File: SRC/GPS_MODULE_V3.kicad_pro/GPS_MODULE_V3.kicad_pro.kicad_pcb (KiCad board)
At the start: 4 copper layers, 53.7 x 41 mm, 143 parts, among them J1 Input, J2 Conn_02x02_Odd_Even, J3 nano_sim, J5 Conn_02x03_Odd_Even, Q1 SSM3J328R-HXY, Q2 BSN20, Q3 BSN20, Q5 2N7002, Q6 2N7002, Q7 2N7002, Q8 2N7002, Q9 2N7002, U1 SY8089AAAC, U2 STM32F103C8Tx, U3 SIM7000E, U4 MAX485E, U7 ATA6561-GAQW-N, U8 W25Q32JVSS, Y1 8MHz, Y2 32.678KHz

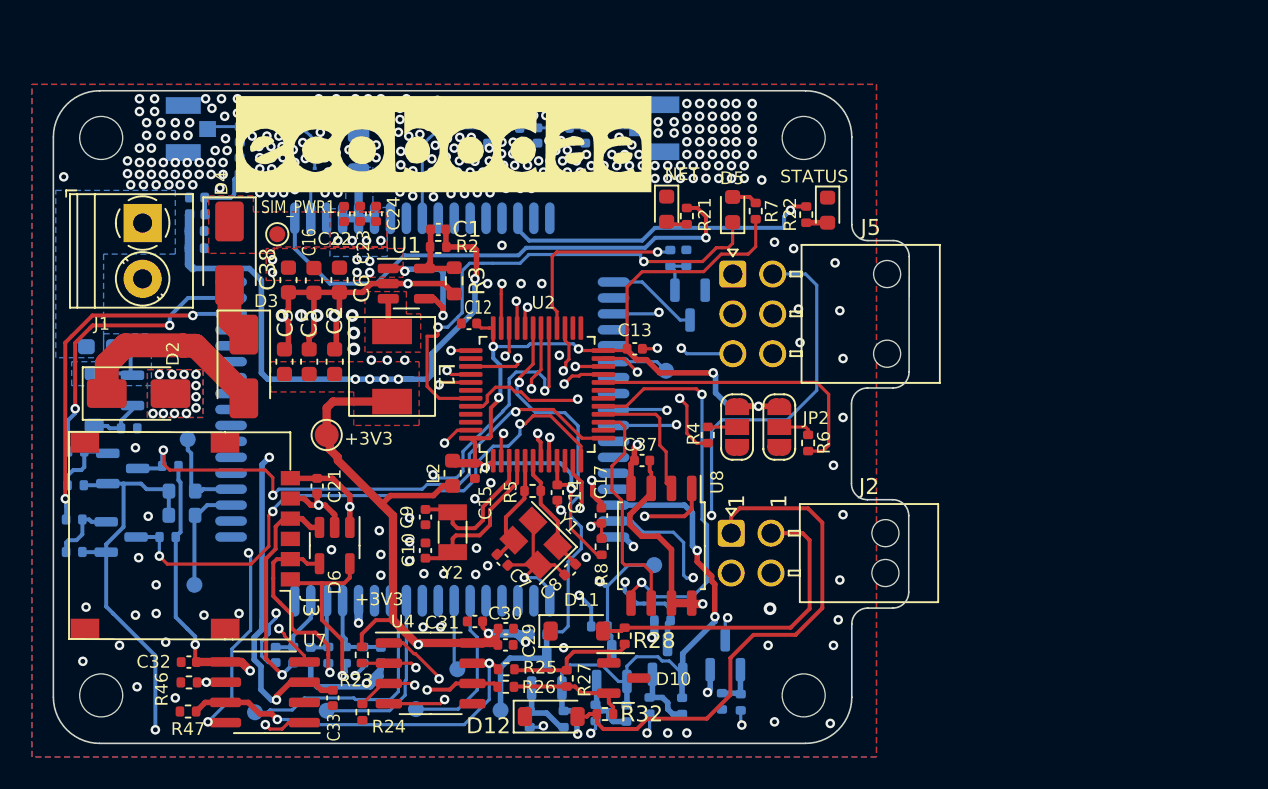
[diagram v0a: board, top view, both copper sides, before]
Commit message: updates on BOM, CPL and gerbers
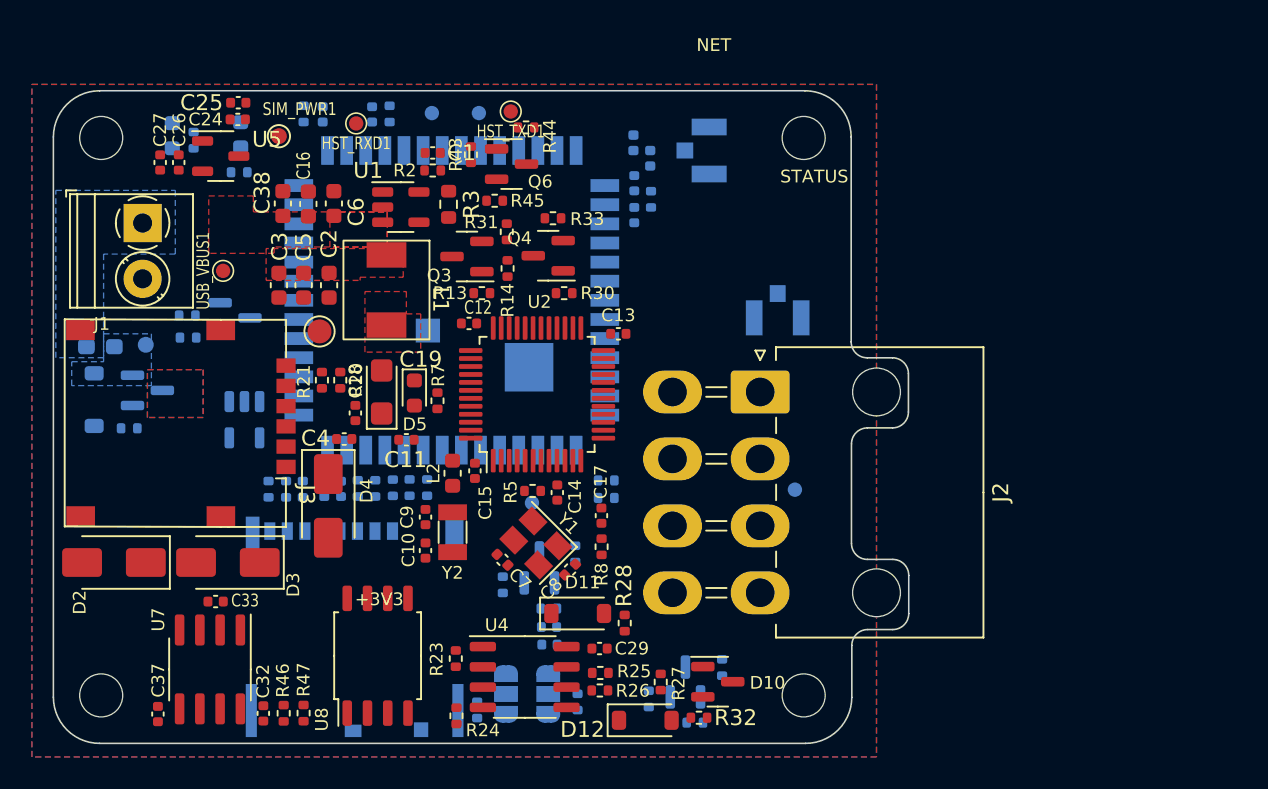
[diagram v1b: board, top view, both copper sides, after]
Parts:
- removed BOOT_CFG1: BOOT_CFG, TestPoint:TestPoint_Pad_D1.0mm
- removed C35: 10n, Capacitor_SMD:C_0402_1005Metric
- removed C36: 1n, Capacitor_SMD:C_0402_1005Metric
- removed FL1: B39162B8813P810, Filter:Filter_1109-5_1.1x0.9mm
- removed the G*** at (247.8, 69.3)
- removed J5: Conn_02x03_Odd_Even, Connector_Molex:Molex_Nano-Fit_105314-xx06_2x03_P2.50mm_Horizontal
- removed L4: 27nH, Inductor_SMD:L_0402_1005Metric
- removed L5: 100mHz 150/200R, Inductor_SMD:L_0402_1005Metric
- removed MDM_LOG_TX1: MDM_LOG_TX, TestPoint:TestPoint_Pad_D1.0mm
- removed Q8, Q9: 2N7002, Package_TO_SOT_SMD:SOT-23
- removed SIM_RX1: Sim_RX, TestPoint:TestPoint_Pad_D1.0mm
- removed SIM_TX1: Sim_TX, TestPoint:TestPoint_Pad_D1.0mm
- added C11: 10u, Capacitor_SMD:C_0402_1005Metric, F.Cu at (245.5, 87.9)
- added C4: 1u, Capacitor_SMD:C_0402_1005Metric, F.Cu at (241.6, 87.8)
- added G***: LOGO, MACHADA_footprints:ECOBODDA_SMALL, B.Cu at (230.8, 97.7)
- added HST_RXD1: HST_RXD, brilliant-kicad-library:TestPoint_Pad_D0.9mm, F.Cu at (242.3, 68.0)
- added HST_TXD1: HST_TXD, brilliant-kicad-library:TestPoint_Pad_D0.9mm, F.Cu at (252.1, 67.3)
- added J4: Micro_SD_Card, MACHADA_footprints:MOLEX_503398-1892, B.Cu at (242.2, 99.2)
- added Q4: 2N7002, Package_TO_SOT_SMD:SOT-23, F.Cu at (254.4, 76.3)
- added R36: 1K, Resistor_SMD:R_0402_1005Metric, B.Cu at (260.7, 104.2)
- added R48: 10K, Resistor_SMD:R_0402_1005Metric, B.Cu at (254.4, 98.5)
- added R49: 10K, Resistor_SMD:R_0402_1005Metric, B.Cu at (256.1, 95.1)
- added R50: 1K, Resistor_SMD:R_0402_1005Metric, B.Cu at (251.6, 97.0)
- added U5: XC6206PxxxMR, Package_TO_SOT_SMD:SOT-23-3, F.Cu at (233.8, 70.1)
- C18: value 22p -> 10u; moved to F.Cu
- C19: value 22p -> 100u; footprint Capacitor_SMD:C_0402_1005Metric -> Capacitor_Tantalum_SMD:CP_EIA-3216-18_Kemet-A; moved to F.Cu
- C20: value 22p -> 1u
- C21: value 100n -> 22p; moved to B.Cu
- C22: value 1u -> 22p; moved to B.Cu
- C23: value 10u -> 22p; moved to B.Cu
- C24: value 10u -> 0.1u
- C25: value 100u -> 1u; footprint Capacitor_Tantalum_SMD:CP_EIA-3216-18_Kemet-A -> Capacitor_SMD:C_0402_1005Metric; moved to F.Cu
- C26: value 0.3p -> 0.1u; moved to F.Cu
- C27: value ~ -> 1u; moved to F.Cu
- C28: value ~ -> 0.1u
- C30, C31, JP1, JP2, R22, R4, R6: moved to B.Cu
- D+1, D-1, SIM_I2C_SCL1, SIM_I2C_SDA1: footprint TestPoint:TestPoint_Pad_D1.0mm -> brilliant-kicad-library:TestPoint_Pad_D0.9mm
- D6: value SP0504BAHT -> LXES15AAA1-153; footprint Package_TO_SOT_SMD:SOT-23-5 -> Diode_SMD:D_0402_1005Metric; moved to B.Cu
- D7: value ORANGE -> SP0504BAHT; footprint LED_SMD:LED_0603_1608Metric -> Package_TO_SOT_SMD:SOT-23-5; moved to B.Cu
- D8: value BLUE -> ORANGE; moved to B.Cu
- D9: value LXES15AAA1-153 -> BLUE; footprint Diode_SMD:D_0402_1005Metric -> LED_SMD:LED_0603_1608Metric
- J2: value Conn_02x02_Odd_Even -> Conn_02x04_Odd_Even; footprint Connector_Molex:Molex_Nano-Fit_105314-xx04_2x02_P2.50mm_Horizontal -> Connector_Molex:Molex_Mini-Fit_Jr_5569-08A2_2x04_P4.20mm_Horizontal
- L3: value 1uH -> 82nH
- Q3, Q6, R43, R44: moved to F.Cu
- R10: value 1k -> 10K
- R12: value 10K -> 1k
- R13: value 22R -> 1k; moved to F.Cu
- R14: value 22R -> 10K; moved to F.Cu
- R15: value 22R -> 2.2K
- R16: value 10K -> 2.2K
- R17, R18: value 2.2K -> 22R; footprint Resistor_SMD:R_0603_1608Metric -> Resistor_SMD:R_0402_1005Metric
- R19: value 0R -> 22R
- R20: value 10R -> 200K; moved to F.Cu
- R21: value 390R -> 100K
- R29: value 1K -> 390R
- R30, R31: value 1K -> 10K; moved to F.Cu
- R33, R45: value 10K -> 1K; moved to F.Cu
- R37, R38, R39, R42: value 10K -> 10k
- R40, R41: value 1K -> 10k
- U3: value SIM7000E -> A9G_MODULE; footprint Lib:SIMCON_SIM7000E -> MACHADA_footprints:A9G_MODULE
- USB_VBUS1: footprint TestPoint:TestPoint_Pad_D1.0mm -> brilliant-kicad-library:TestPoint_Pad_D0.9mm; moved to F.Cu
- moved R10 42.4 mm to (231.8, 80.1), turned to 0 degrees
- moved D8 41.4 mm to (230.8, 68.8)
- moved R29 40.6 mm to (235.0, 71.1), turned to 180 degrees
- moved D-1 40.1 mm to (250.1, 67.4), turned to 90 degrees
- moved AE2 39.1 mm to (268.8, 80.2), turned to 0 degrees
- moved R22 38.7 mm to (232.2, 69.1)
- moved SIM_I2C_SDA1 38.2 mm to (269.9, 91.0)
- moved D+1 38.1 mm to (247.1, 67.4), turned to 90 degrees
- moved C20 35.6 mm to (259.8, 73.8)
- moved R17 34.7 mm to (260.9, 72.8), turned to -90 degrees
- moved C37 34.3 mm to (229.9, 105.1), turned to -90 degrees
- moved R44 34.2 mm to (253.0, 68.3), turned to 0 degrees
- moved Q6 32.6 mm to (252.1, 70.6), turned to 0 degrees
- moved R43 32.3 mm to (249.6, 70.0), turned to -90 degrees
- moved R33 31.4 mm to (254.7, 74.0), turned to 0 degrees
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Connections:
- C18 pad 1: /SIM7000E_GPRS_SIM MODULE/Sim_DIO -> 4.2V_SIMPWR
- C19 pad 1: /SIM7000E_GPRS_SIM MODULE/Sim_CLK -> 4.2V_SIMPWR
- C20 pad 1: /SIM7000E_GPRS_SIM MODULE/Sim_RST -> /A9G_GSM_GPRS_MODULE/VIO
- C21 pad 1: /SIM7000E_GPRS_SIM MODULE/V_Sim -> /A9G_GSM_GPRS_MODULE/Sim_DIO
- C22 pad 1: 4.2V_SIMPWR -> /A9G_GSM_GPRS_MODULE/Sim_CLK
- C23 pad 1: 4.2V_SIMPWR -> /A9G_GSM_GPRS_MODULE/Sim_RST
- C26 pad 1: GND -> 2V8
- C26 pad 2: /SIM7000E_GPRS_SIM MODULE/RF_ANT -> GND
- C27 pad 1: GND -> 2V8
- C27 pad 2: Net-(C27-Pad2) -> GND
- C28 pad 1: GND -> /A9G_GSM_GPRS_MODULE/TF_CARD_CONN/2V8
- C28 pad 2: Net-(AE1-A) -> GND
- C34 pad 1: +3V3 -> /A9G_GSM_GPRS_MODULE/TF_CARD_CONN/2V8
- D+1 pad 1: Net-(U3-USB_DP) -> Net-(U3-USB_P)
- D-1 pad 1: Net-(U3-USB_DM) -> Net-(U3-USB_N)
- D6 pad 1: /SIM7000E_GPRS_SIM MODULE/V_Sim -> GND
- D6 pad 2: GND -> Net-(AE1-A)
- D7 pad 1: GND -> /A9G_GSM_GPRS_MODULE/V_Sim
- D7 pad 2: Net-(D7-A) -> GND
- D9 pad 2: Net-(AE1-A) -> Net-(D9-A)
- J2 pad 1: /RS485_MAX485/A -> GND
- J2 pad 3: /RS485_MAX485/B -> /RS485_MAX485/A
- J2 pad 4: GND -> /STM32F103C8T6_MCU/SW0
- J3 pad C1: /SIM7000E_GPRS_SIM MODULE/V_Sim -> /A9G_GSM_GPRS_MODULE/V_Sim
- L3 pad 1: /SIM7000E_GPRS_SIM MODULE/RF_ANT -> GND
- L3 pad 2: Net-(C27-Pad2) -> Net-(AE1-A)
- Q5 pad 1: /SIM7000E_GPRS_SIM MODULE/VDD_EXT -> 2V8
- Q5 pad 3: /STM32F103C8T6_MCU/TX1 -> /STM32F103C8T6_MCU/RX2
- Q6 pad 1: /SIM7000E_GPRS_SIM MODULE/VDD_EXT -> 2V8
- Q6 pad 3: /SIM7000E_GPRS_SIM MODULE/SIM_DTR -> /STM32F103C8T6_MCU/TX2
- Q7 pad 1: /SIM7000E_GPRS_SIM MODULE/VDD_EXT -> 2V8
- Q7 pad 3: /STM32F103C8T6_MCU/RX1 -> /STM32F103C8T6_MCU/TX1
- R10 pad 1: /SIM7000E_GPRS_SIM MODULE/Sim_Reset -> GND
- R10 pad 2: Net-(Q3-G) -> Net-(Q2-G)
- R11 pad 1: GND -> Net-(Q3-D)
- R11 pad 2: Net-(Q2-G) -> /A9G_GSM_GPRS_MODULE/VIO
- R12 pad 1: GND -> /A9G_GSM_GPRS_MODULE/IO29
- R12 pad 2: Net-(Q3-G) -> Net-(Q3-D)
- R13 pad 1: /SIM7000E_GPRS_SIM MODULE/Sim_RST -> /A9G_GSM_GPRS_MODULE/PWRKEY
- R13 pad 2: Net-(J3-RST) -> Net-(Q3-G)
- R14 pad 1: /SIM7000E_GPRS_SIM MODULE/Sim_CLK -> GND
- R14 pad 2: Net-(J3-CLK) -> Net-(Q3-G)
- R15 pad 1: /SIM7000E_GPRS_SIM MODULE/Sim_DIO -> Net-(U3-I2C2_SCL/IO19)
- R15 pad 2: Net-(J3-I/O) -> /A9G_GSM_GPRS_MODULE/VIO
- R16 pad 1: /SIM7000E_GPRS_SIM MODULE/Sim_DIO -> Net-(U3-I2C2_SDA/IO20)
- R16 pad 2: /SIM7000E_GPRS_SIM MODULE/V_Sim -> /A9G_GSM_GPRS_MODULE/VIO
- R17 pad 1: Net-(U3-I2C_SCL) -> /A9G_GSM_GPRS_MODULE/Sim_RST
- R17 pad 2: /SIM7000E_GPRS_SIM MODULE/VDD_EXT -> Net-(J3-RST)
- R18 pad 1: Net-(U3-I2C_SDA) -> /A9G_GSM_GPRS_MODULE/Sim_CLK
- R18 pad 2: /SIM7000E_GPRS_SIM MODULE/VDD_EXT -> Net-(J3-CLK)
- R19 pad 1: Net-(C27-Pad2) -> /A9G_GSM_GPRS_MODULE/Sim_DIO
- R19 pad 2: Net-(AE1-A) -> Net-(J3-I/O)
- R20 pad 1: Net-(L4-Pad1) -> Net-(U3-ADC0)
- R20 pad 2: /SIM7000E_GPRS_SIM MODULE/gps_VDD -> 4.2V_SIMPWR
- R21 pad 1: /SIM7000E_GPRS_SIM MODULE/NETLIGHT -> GND
- R21 pad 2: Net-(D7-A) -> Net-(U3-ADC0)
- R22 pad 1: /SIM7000E_GPRS_SIM MODULE/STATUS -> /A9G_GSM_GPRS_MODULE/GPRS_NET-STATUS
- R29 pad 1: /SIM7000E_GPRS_SIM MODULE/MOSFET_LOGIC_LEVEL_TRANSLATOR/LOW_SIDE_SIM_RXD_LOGIC -> /A9G_GSM_GPRS_MODULE/GPS POSITION
- R29 pad 2: Net-(Q5-S) -> Net-(D9-A)
- R30 pad 1: /SIM7000E_GPRS_SIM MODULE/MOSFET_LOGIC_LEVEL_TRANSLATOR/LOW_SIDE_SIM_DTR_LOGIC -> 2V8
- R30 pad 2: Net-(Q6-S) -> Net-(Q4-S)
- R31 pad 1: /SIM7000E_GPRS_SIM MODULE/MOSFET_LOGIC_LEVEL_TRANSLATOR/LOW_SIDE_SIM_TXD_LOGIC -> +3V3
- R31 pad 2: Net-(Q7-S) -> /STM32F103C8T6_MCU/RX1
- R33 pad 1: /SIM7000E_GPRS_SIM MODULE/VDD_EXT -> /A9G_GSM_GPRS_MODULE/MOSFET_LOGIC_LEVEL_TRANSLATOR9/LOW_SIDE_LOGIC_SIGNAL
- R33 pad 2: Net-(Q5-S) -> Net-(Q4-S)
- R34 pad 1: /SIM7000E_GPRS_SIM MODULE/VDD_EXT -> 2V8
- R34 pad 2: Net-(Q6-S) -> Net-(Q5-S)
- R35 pad 1: /SIM7000E_GPRS_SIM MODULE/VDD_EXT -> +3V3
- R35 pad 2: Net-(Q7-S) -> /STM32F103C8T6_MCU/RX2
- R37 pad 1: +3V3 -> /A9G_GSM_GPRS_MODULE/TF_CARD_CONN/2V8
- R37 pad 2: /STM32F103C8T6_MCU/TX1 -> /A9G_GSM_GPRS_MODULE/TF_CARD_CONN/SD_D2
- R38 pad 1: +3V3 -> /A9G_GSM_GPRS_MODULE/TF_CARD_CONN/2V8
- R38 pad 2: /SIM7000E_GPRS_SIM MODULE/SIM_DTR -> /A9G_GSM_GPRS_MODULE/TF_CARD_CONN/SD_D3
- R39 pad 1: +3V3 -> /A9G_GSM_GPRS_MODULE/TF_CARD_CONN/2V8
- R39 pad 2: /STM32F103C8T6_MCU/RX1 -> /A9G_GSM_GPRS_MODULE/TF_CARD_CONN/SD_CMD
- R40 pad 1: /SIM7000E_GPRS_SIM MODULE/GPS_RXD_ -> /A9G_GSM_GPRS_MODULE/TF_CARD_CONN/2V8
- R40 pad 2: Net-(Q8-S) -> /A9G_GSM_GPRS_MODULE/TF_CARD_CONN/SD_D0
- R41 pad 1: /SIM7000E_GPRS_SIM MODULE/GPS_TXD_ -> /A9G_GSM_GPRS_MODULE/TF_CARD_CONN/2V8
- R41 pad 2: Net-(Q9-S) -> /A9G_GSM_GPRS_MODULE/TF_CARD_CONN/SD_D1
- R42 pad 1: /SIM7000E_GPRS_SIM MODULE/VDD_EXT -> /A9G_GSM_GPRS_MODULE/TF_CARD_CONN/2V8
- R42 pad 2: Net-(Q8-S) -> /A9G_GSM_GPRS_MODULE/TF_CARD_CONN/SD_CLK
- R43 pad 1: /SIM7000E_GPRS_SIM MODULE/VDD_EXT -> 2V8
- R43 pad 2: Net-(Q9-S) -> Net-(Q6-S)
- R45 pad 1: +3V3 -> /A9G_GSM_GPRS_MODULE/MOSFET_LOGIC_LEVEL_TRANSLATOR7/LOW_SIDE_LOGIC_SIGNAL
- R45 pad 2: /STM32F103C8T6_MCU/RX2 -> Net-(Q6-S)
- R9 pad 1: /SIM7000E_GPRS_SIM MODULE/PWRKEY -> /A9G_GSM_GPRS_MODULE/Sim_Restart
- SIM_I2C_SCL1 pad 1: Net-(U3-I2C_SCL) -> Net-(U3-I2C2_SCL/IO19)
- SIM_I2C_SDA1 pad 1: Net-(U3-I2C_SDA) -> Net-(U3-I2C2_SDA/IO20)
- U2 pad 28: /SIM7000E_GPRS_SIM MODULE/PWRKEY -> /A9G_GSM_GPRS_MODULE/PWRKEY
- U2 pad 40: /SIM7000E_GPRS_SIM MODULE/Sim_Reset -> /A9G_GSM_GPRS_MODULE/Sim_Restart
- U2 pad 41: /SIM7000E_GPRS_SIM MODULE/SIM_DTR -> /STM32F103C8T6_MCU/Sim_DTR
- U3 pad 1: Net-(Q2-D) -> Net-(U3-I2C2_SCL/IO19)
- U3 pad 10: /SIM7000E_GPRS_SIM MODULE/MOSFET_LOGIC_LEVEL_TRANSLATOR/LOW_SIDE_SIM_RXD_LOGIC -> GND
- U3 pad 11: unconnected-(U3-PCM_CLK-Pad11) -> 4.2V_SIMPWR
- U3 pad 12: unconnected-(U3-PCM_SYNC-Pad12) -> 4.2V_SIMPWR
- U3 pad 15: /SIM7000E_GPRS_SIM MODULE/VDD_EXT -> Net-(U3-ADC0)
- U3 pad 16: Net-(Q3-D) -> unconnected-(U3-ADC1-Pad16)
- U3 pad 17: GND -> Net-(U3-VUSB_DET)
- U3 pad 18: GND -> Net-(Q2-D)
- U3 pad 19: (no net) -> unconnected-(U3-LCD_CS/I2S_LRCK/IO15-Pad19)
- U3 pad 2: GND -> Net-(U3-I2C2_SDA/IO20)
- U3 pad 20: (no net) -> unconnected-(U3-LCD_RSTB/I2S_BCK/IO14-Pad20)
- U3 pad 21: (no net) -> unconnected-(U3-LCD_DIO/I2S_DO/IO17-Pad21)
- U3 pad 22: (no net) -> unconnected-(U3-LCD_DC/IO18-Pad22)
- U3 pad 23: Net-(U3-MDM_LOG_TX) -> unconnected-(U3-LCD_SCK/I2S_DI/IO16-Pad23)
- U3 pad 24: Net-(U3-USB_VBUS) -> /A9G_GSM_GPRS_MODULE/IO29
- U3 pad 26: (no net) -> /A9G_GSM_GPRS_MODULE/GPRS_NET-STATUS
- U3 pad 27: Net-(U3-USB_DP) -> GND
- U3 pad 28: Net-(U3-USB_DM) -> /A9G_GSM_GPRS_MODULE/Sim_CLK
- U3 pad 29: GND -> /A9G_GSM_GPRS_MODULE/V_Sim
- U3 pad 3: /SIM7000E_GPRS_SIM MODULE/MOSFET_LOGIC_LEVEL_TRANSLATOR/LOW_SIDE_SIM_DTR_LOGIC -> /A9G_GSM_GPRS_MODULE/TF_CARD_CONN/SD_D3
- U3 pad 30: /SIM7000E_GPRS_SIM MODULE/V_Sim -> /A9G_GSM_GPRS_MODULE/Sim_DIO
- U3 pad 31: /SIM7000E_GPRS_SIM MODULE/Sim_DIO -> Net-(U3-HST_RXD)
- U3 pad 32: /SIM7000E_GPRS_SIM MODULE/Sim_CLK -> Net-(U3-HST_TXD)
- U3 pad 33: /SIM7000E_GPRS_SIM MODULE/Sim_RST -> Net-(U3-USB_P)
- U3 pad 34: /SIM7000E_GPRS_SIM MODULE/Sim_DET -> Net-(U3-USB_N)
- U3 pad 35: (no net) -> unconnected-(U3-MIC_P-Pad35)
- U3 pad 36: (no net) -> unconnected-(U3-MIC_N-Pad36)
- U3 pad 37: Net-(U3-I2C_SDA) -> unconnected-(U3-IO25-Pad37)
- U3 pad 38: Net-(U3-I2C_SCL) -> unconnected-(U3-IO30-Pad38)
- U3 pad 39: GND -> /A9G_GSM_GPRS_MODULE/GPS POSITION
- U3 pad 4: unconnected-(U3-RI-Pad4) -> /A9G_GSM_GPRS_MODULE/TF_CARD_CONN/SD_D2
- U3 pad 40: (no net) -> GND
- U3 pad 41: (no net) -> Net-(AE1-A)
- U3 pad 42: (no net) -> /A9G_GSM_GPRS_MODULE/Sim_RST
- U3 pad 43: (no net) -> /A9G_GSM_GPRS_MODULE/VIO
- U3 pad 44: (no net) -> GND
- U3 pad 45: GND -> Net-(AE2-A)
- U3 pad 46: GND -> unconnected-(U3-GND-Pad46)
- U3 pad 47: (no net) -> unconnected-(U3-UART2_RTS/I2C3_SDA/IO7-Pad47)
- U3 pad 49: /SIM7000E_GPRS_SIM MODULE/GPS_RXD_ -> /A9G_GSM_GPRS_MODULE/MOSFET_LOGIC_LEVEL_TRANSLATOR7/LOW_SIDE_LOGIC_SIGNAL
- U3 pad 5: unconnected-(U3-DCD-Pad5) -> /A9G_GSM_GPRS_MODULE/TF_CARD_CONN/SD_D1
- U3 pad 50: /SIM7000E_GPRS_SIM MODULE/GPS_TXD_ -> /A9G_GSM_GPRS_MODULE/MOSFET_LOGIC_LEVEL_TRANSLATOR6/LOW_SIDE_LOGIC_SIGNAL
- U3 pad 51: (no net) -> unconnected-(U3-UART1_RTS/IO3-Pad51)
- U3 pad 52: /SIM7000E_GPRS_SIM MODULE/NETLIGHT -> unconnected-(U3-UART1_CTS/IO2-Pad52)
- U3 pad 53: /SIM7000E_GPRS_SIM MODULE/GNSS_ANT -> /A9G_GSM_GPRS_MODULE/MOSFET_LOGIC_LEVEL_TRANSLATOR8/LOW_SIDE_LOGIC_SIGNAL
- U3 pad 54: GND -> /A9G_GSM_GPRS_MODULE/MOSFET_LOGIC_LEVEL_TRANSLATOR9/LOW_SIDE_LOGIC_SIGNAL
- U3 pad 55: 4.2V_SIMPWR -> GND
- U3 pad 56: 4.2V_SIMPWR -> GND
- U3 pad 6: Net-(U3-BOOT_CFG) -> /A9G_GSM_GPRS_MODULE/TF_CARD_CONN/SD_D0
- U3 pad 7: unconnected-(U3-CTS-Pad7) -> /A9G_GSM_GPRS_MODULE/TF_CARD_CONN/SD_CMD
- U3 pad 8: unconnected-(U3-RTS-Pad8) -> /A9G_GSM_GPRS_MODULE/TF_CARD_CONN/SD_CLK
- U3 pad 9: /SIM7000E_GPRS_SIM MODULE/MOSFET_LOGIC_LEVEL_TRANSLATOR/LOW_SIDE_SIM_TXD_LOGIC -> Net-(Q3-D)
- USB_VBUS1 pad 1: Net-(U3-USB_VBUS) -> Net-(U3-VUSB_DET)
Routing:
- net +3V3: track 142.6 -> 0.00 mm, vias 13 -> 0
- net /SIM7000E_GPRS_SIM MODULE/VDD_EXT: track 86.8 -> 0.00 mm, vias 4 -> 0
- net +5V: track 78.1 -> 0.00 mm, vias 21 -> 0
- net GND: track 69.3 -> 0.00 mm, vias 382 -> 0
- net /STM32F103C8T6_MCU/3v3_stm: track 65.2 -> 0.00 mm, vias 7 -> 0
- net /CAN_TRANSCEIVER_ATA6561/CAN_TX: track 47.4 -> 0.00 mm, vias 2 -> 0
- net /CAN_TRANSCEIVER_ATA6561/CAN_STBY: track 45.2 -> 0.00 mm, vias 4 -> 0
- net /STM32F103C8T6_MCU/mcu_reset: track 43.8 -> 0.00 mm, vias 3 -> 0
- net /SIM7000E_GPRS_SIM MODULE/Sim_Reset: track 43.4 -> 0.00 mm, vias 3 -> 0
- net /STM32F103C8T6_MCU/TX3: track 43.3 -> 0.00 mm, vias 2 -> 0
- net /STM32F103C8T6_MCU/RX3: track 43.2 -> 0.00 mm, vias 2 -> 0
- net /RS485_MAX485/RS485_DE: track 40.8 -> 0.00 mm, vias 2 -> 0
- net /CAN_TRANSCEIVER_ATA6561/CAN_RX: track 38.8 -> 0.00 mm, vias 2 -> 0
- net /RS485_MAX485/RS485_~{RE}: track 37.2 -> 0.00 mm, vias 2 -> 0
- net /STM32F103C8T6_MCU/TX2: track 37.0 -> 0.00 mm, vias 3 -> 0
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- removed copper zone on F.Cu, net +3V3
- removed copper zone on B.Cu, net 4.2V_SIMPWR
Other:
- outline, holes or cut-outs redrawn

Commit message: routing
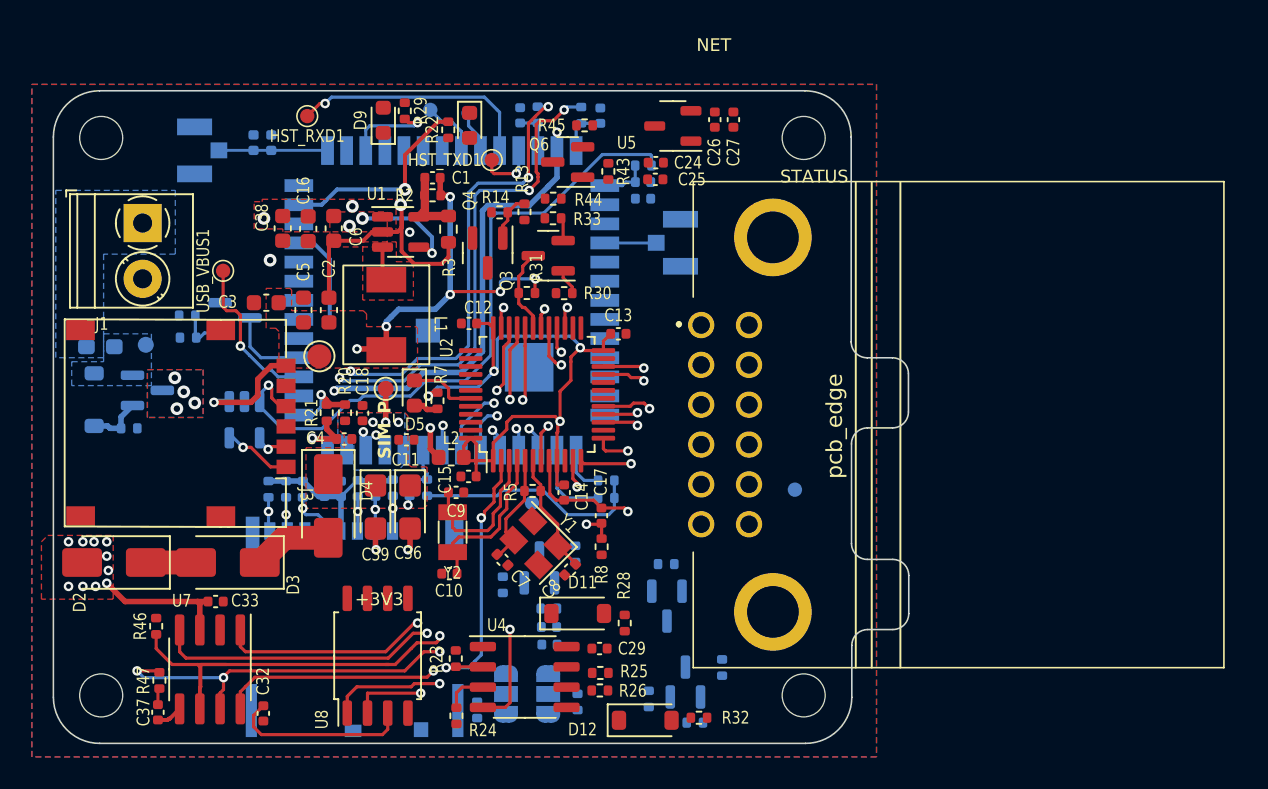
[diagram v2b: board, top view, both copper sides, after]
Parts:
- removed C19: 100u, Capacitor_Tantalum_SMD:CP_EIA-3216-18_Kemet-A
- removed J2: Conn_02x04_Odd_Even, Connector_Molex:Molex_Mini-Fit_Jr_5569-08A2_2x04_P4.20mm_Horizontal
- added C36: 100u, Capacitor_Tantalum_SMD:CP_EIA-3216-18_Kemet-A, F.Cu at (245.7, 92.1)
- added C39: 100u, Capacitor_Tantalum_SMD:CP_EIA-3216-18_Kemet-A, F.Cu at (243.6, 92.1)
- added J5: Conn_02x06_Counter_Clockwise, MACHADA_footprints:auto_jae_conn_02x06_p2.5mm_MX23A12NF1, F.Cu at (279.6, 87.0)
- D10, H3, H4, R27: moved to B.Cu
- D8, D9, R22, R29: moved to F.Cu
- moved C27 36.1 mm to (266.0, 67.8), turned to -90 degrees
- moved C26 33.7 mm to (264.9, 67.8), turned to -90 degrees
- moved AE1 32.3 mm to (232.2, 69.7), turned to -90 degrees
- moved U5 28.4 mm to (262.2, 68.2), turned to 180 degrees
- moved C25 26.6 mm to (261.1, 71.6), turned to 0 degrees
- moved C24 26.4 mm to (261.1, 70.5), turned to 0 degrees
- moved D6 24.9 mm to (235.9, 69.3), turned to -90 degrees
- moved L3 22.7 mm to (237.0, 69.3)
- moved D8 18.7 mm to (249.5, 68.2)
- moved C22 17.4 mm to (257.7, 67.6)
- moved R18 17.4 mm to (256.5, 67.5)
- moved SIM_PWR1 17.2 mm to (244.2, 84.7), turned to 90 degrees
- moved R22 16.0 mm to (248.1, 68.5)
- moved R29 11.1 mm to (245.4, 67.3), turned to 90 degrees
- moved R46 9.69 mm to (229.8, 99.6), turned to 90 degrees
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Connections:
- C28 pad 1: /A9G_GSM_GPRS_MODULE/TF_CARD_CONN/2V8 -> 2V8
- C34 pad 1: /A9G_GSM_GPRS_MODULE/TF_CARD_CONN/2V8 -> 2V8
- HST_RXD1 pad 1: Net-(U3-HST_RXD) -> Net-(U3-HST_TXD)
- HST_TXD1 pad 1: Net-(U3-HST_TXD) -> Net-(U3-HST_RXD)
- J4 pad 4: /A9G_GSM_GPRS_MODULE/TF_CARD_CONN/2V8 -> 2V8
- R37 pad 1: /A9G_GSM_GPRS_MODULE/TF_CARD_CONN/2V8 -> 2V8
- R38 pad 1: /A9G_GSM_GPRS_MODULE/TF_CARD_CONN/2V8 -> 2V8
- R39 pad 1: /A9G_GSM_GPRS_MODULE/TF_CARD_CONN/2V8 -> 2V8
- R40 pad 1: /A9G_GSM_GPRS_MODULE/TF_CARD_CONN/2V8 -> 2V8
- R41 pad 1: /A9G_GSM_GPRS_MODULE/TF_CARD_CONN/2V8 -> 2V8
- R42 pad 1: /A9G_GSM_GPRS_MODULE/TF_CARD_CONN/2V8 -> 2V8
- U3 pad 28: /A9G_GSM_GPRS_MODULE/Sim_CLK -> Net-(AE1-A)
- U3 pad 29: /A9G_GSM_GPRS_MODULE/V_Sim -> GND
- U3 pad 30: /A9G_GSM_GPRS_MODULE/Sim_DIO -> /A9G_GSM_GPRS_MODULE/GPS POSITION
- U3 pad 31: Net-(U3-HST_RXD) -> unconnected-(U3-IO30-Pad31)
- U3 pad 32: Net-(U3-HST_TXD) -> unconnected-(U3-IO25-Pad32)
- U3 pad 33: Net-(U3-USB_P) -> unconnected-(U3-MIC_N-Pad33)
- U3 pad 34: Net-(U3-USB_N) -> unconnected-(U3-MIC_P-Pad34)
- U3 pad 35: unconnected-(U3-MIC_P-Pad35) -> Net-(U3-USB_N)
- U3 pad 36: unconnected-(U3-MIC_N-Pad36) -> Net-(U3-USB_P)
- U3 pad 37: unconnected-(U3-IO25-Pad37) -> Net-(U3-HST_TXD)
- U3 pad 38: unconnected-(U3-IO30-Pad38) -> Net-(U3-HST_RXD)
- U3 pad 39: /A9G_GSM_GPRS_MODULE/GPS POSITION -> /A9G_GSM_GPRS_MODULE/Sim_DIO
- U3 pad 40: GND -> /A9G_GSM_GPRS_MODULE/V_Sim
- U3 pad 41: Net-(AE1-A) -> /A9G_GSM_GPRS_MODULE/Sim_CLK
- U3 pad 46: unconnected-(U3-GND-Pad46) -> GND
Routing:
- net +3V3: track 0.00 -> 48.5 mm, vias 0 -> 7
- net /A9G_GSM_GPRS_MODULE/V_Sim: track 0.00 -> 43.0 mm, vias 0 -> 3
- net /STM32F103C8T6_MCU/3v3_stm: track 0.00 -> 42.3 mm, vias 0 -> 4
- net Net-(J3-I/O): track 0.00 -> 41.7 mm, vias 0 -> 4
- net Net-(J3-RST): track 0.00 -> 41.5 mm, vias 0 -> 1
- net Net-(J3-CLK): track 0.00 -> 40.5 mm, vias 0 -> 4
- net GND: track 0.00 -> 31.9 mm, vias 0 -> 8
- net A_to_CANL: track 0.00 -> 27.4 mm, vias 0 -> 1
- net /A9G_GSM_GPRS_MODULE/TF_CARD_CONN/SD_CLK: track 0.00 -> 25.5 mm, vias 0 -> 2
- net /A9G_GSM_GPRS_MODULE/TF_CARD_CONN/SD_CMD: track 0.00 -> 25.4 mm, vias 0 -> 2
- net /A9G_GSM_GPRS_MODULE/TF_CARD_CONN/SD_D0: track 0.00 -> 24.0 mm, vias 0 -> 2
- net B_to_CANH: track 0.00 -> 23.4 mm, vias 0 -> 3
- net /CAN_TRANSCEIVER_ATA6561/CAN_RX: track 0.00 -> 22.4 mm, vias 0 -> 2
- net /A9G_GSM_GPRS_MODULE/TF_CARD_CONN/SD_D1: track 0.00 -> 21.9 mm, vias 0 -> 2
- net /A9G_GSM_GPRS_MODULE/TF_CARD_CONN/SD_D3: track 0.00 -> 18.0 mm, vias 0 -> 2
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- added copper zone on F.Cu, net +3V3
- added copper zone on B.Cu, net 4.2V_SIMPWR
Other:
- board text added: "SIM_P"

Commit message: completed GPS
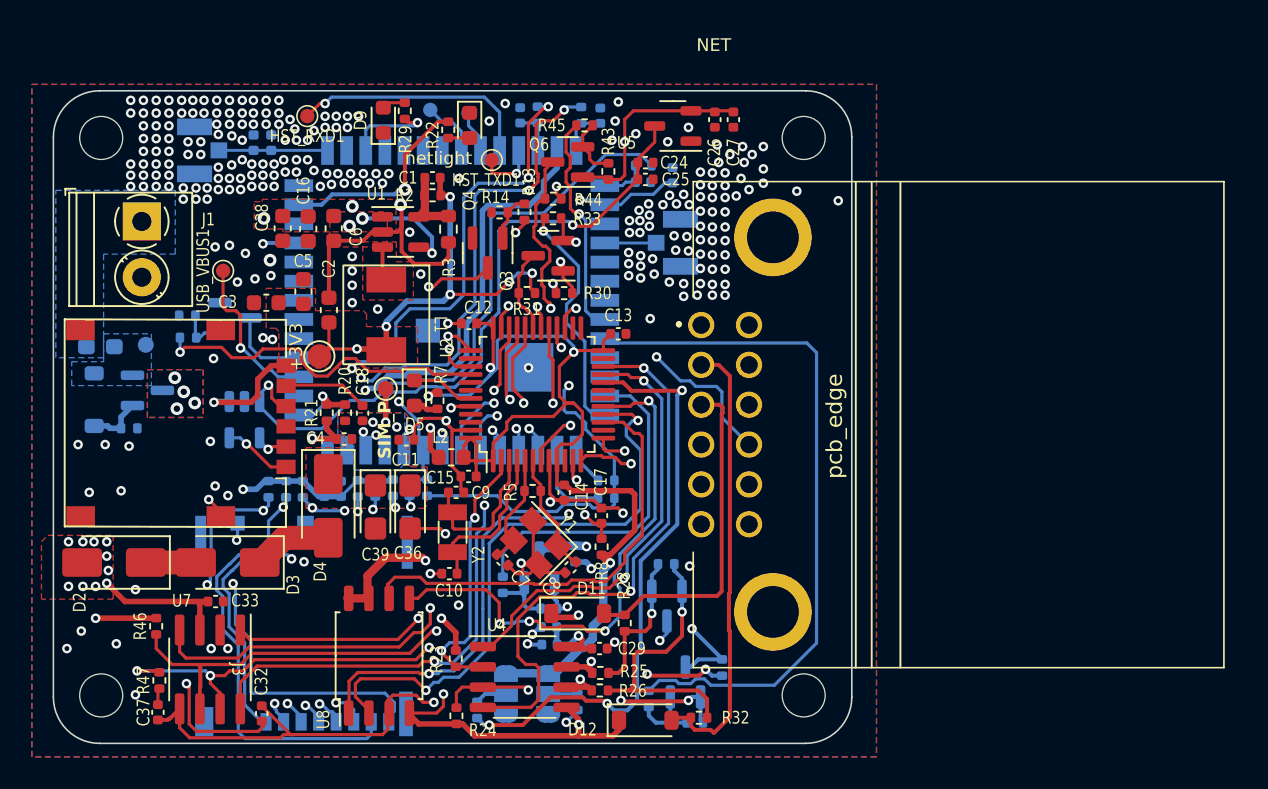
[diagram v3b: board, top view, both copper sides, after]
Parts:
- removed SIM_I2C_SCL1: SIM_I2C_SCL, brilliant-kicad-library:TestPoint_Pad_D0.9mm
- removed SIM_I2C_SDA1: SIM_I2C_SDA, brilliant-kicad-library:TestPoint_Pad_D0.9mm
- moved J4 3.26 mm to (239.1, 100.0), turned to 0 degrees
- moved C20 2.36 mm to (262.2, 71.3), turned to 90 degrees
- moved C5 1.16 mm to (239.0, 78.6)
- moved C24 0.65 mm to (260.5, 70.5)
- moved C25 0.62 mm to (260.5, 71.6)
- moved G*** 0.51 mm to (230.3, 97.7)
- moved C8 0.15 mm to (255.8, 95.9)
- moved J1 0.11 mm to (228.9, 74.2)
- moved C32 0.10 mm to (236.4, 105.1)
- moved U8 0.09 mm to (243.8, 101.5)
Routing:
- net 2V8: track 12.5 -> 150.0 mm, vias 0 -> 8
- net +3V3: track 48.5 -> 129.9 mm, vias 7 -> 15
- net +5V: track 15.5 -> 90.6 mm
- net GND: track 31.9 -> 102.1 mm, vias 8 -> 253
- net /RS485_MAX485/RS485_DE: track 4.09 -> 51.9 mm, vias 1 -> 2
- net /A9G_GSM_GPRS_MODULE/MOSFET_LOGIC_LEVEL_TRANSLATOR6/LOW_SIDE_LOGIC_SIGNAL: track 0.00 -> 44.1 mm
- net /STM32F103C8T6_MCU/BOOT1: track 0.00 -> 37.3 mm, vias 0 -> 3
- net /A9G_GSM_GPRS_MODULE/IO29: track 6.77 -> 42.6 mm, vias 1 -> 2
- net /A9G_GSM_GPRS_MODULE/VIO: track 14.5 -> 47.2 mm, vias 0 -> 3
- net /STM32F103C8T6_MCU/TX1: track 1.32 -> 33.6 mm, vias 1 -> 2
- net 4.2V_SIMPWR: track 2.10 -> 33.9 mm, vias 5 -> 6
- net /FLASH_MEMORY/MISO: track 6.77 -> 37.8 mm
- net /FLASH_MEMORY/MOSI: track 3.12 -> 33.8 mm, vias 1 -> 4
- net /STM32F103C8T6_MCU/SW0: track 0.00 -> 29.6 mm, vias 0 -> 1
- net /RS485_MAX485/A: track 0.00 -> 28.4 mm
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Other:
- board size 53.7 x 41 mm -> 50.1 x 41 mm
- board text added: "netlight"
- board text added: "pwr in"
